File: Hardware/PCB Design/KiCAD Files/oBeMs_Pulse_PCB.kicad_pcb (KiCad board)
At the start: 2 copper layers, 180.3 x 120.7 mm, 132 parts, among them P1 1WIRE_OUT, P10 5V, P11 3V3, P12 GND, P13 ADC_0-7, P14 ADC_8-15, P15 ADC_VREF_2, P16 ADC_VREF_1, P17 SPI_ADC_DAC, P18 DIO_OUTPUT, P19 PULL_UP, P2 1WIRE_SENSOR, P20 PULL_DOWN, P21 DIO_INPUT, P22 DIO_OUTPUT, P23 PULL_UP, P24 PULL_DOWN, P25 DIO_INPUT, P26 DIO_OUTPUT, P27 PULL_UP, P28 PULL_DOWN, P29 DIO_INPUT, P3 HARD_WDT, P34 DAC_A, P35 DAC_B, P36 PROTOTYPING_AREA, P4 LED 5-8, P6 AC_INPUT, P7 LED 1-4, P8 VIN_DC, Q1 BC546, Q2 BC556, U1 LM2575, U2 DS18B20, U3 TLC555, U4 4017, U5 MCP3008, U6 MCP3008, U7 MCP4802, U8 LM2576

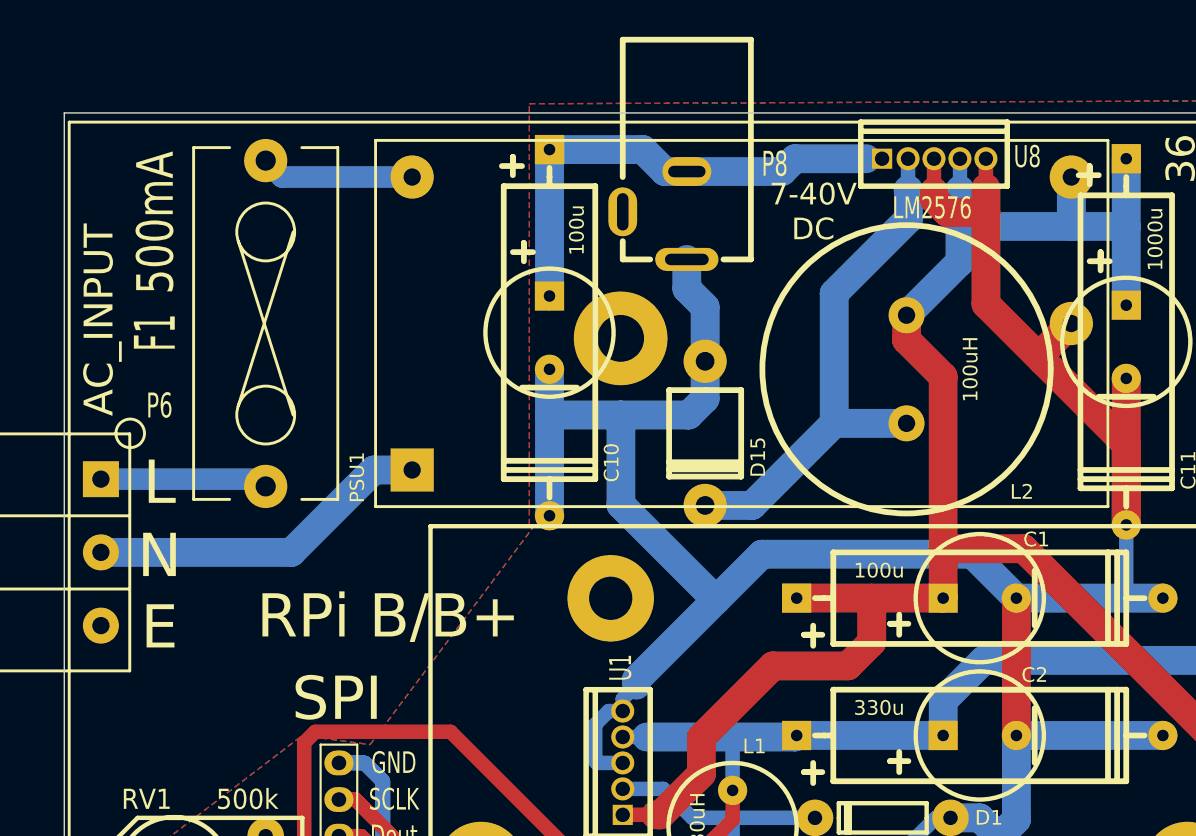
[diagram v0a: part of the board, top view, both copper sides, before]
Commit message: Updated small changes.
Info and changes from email 18/12/15.
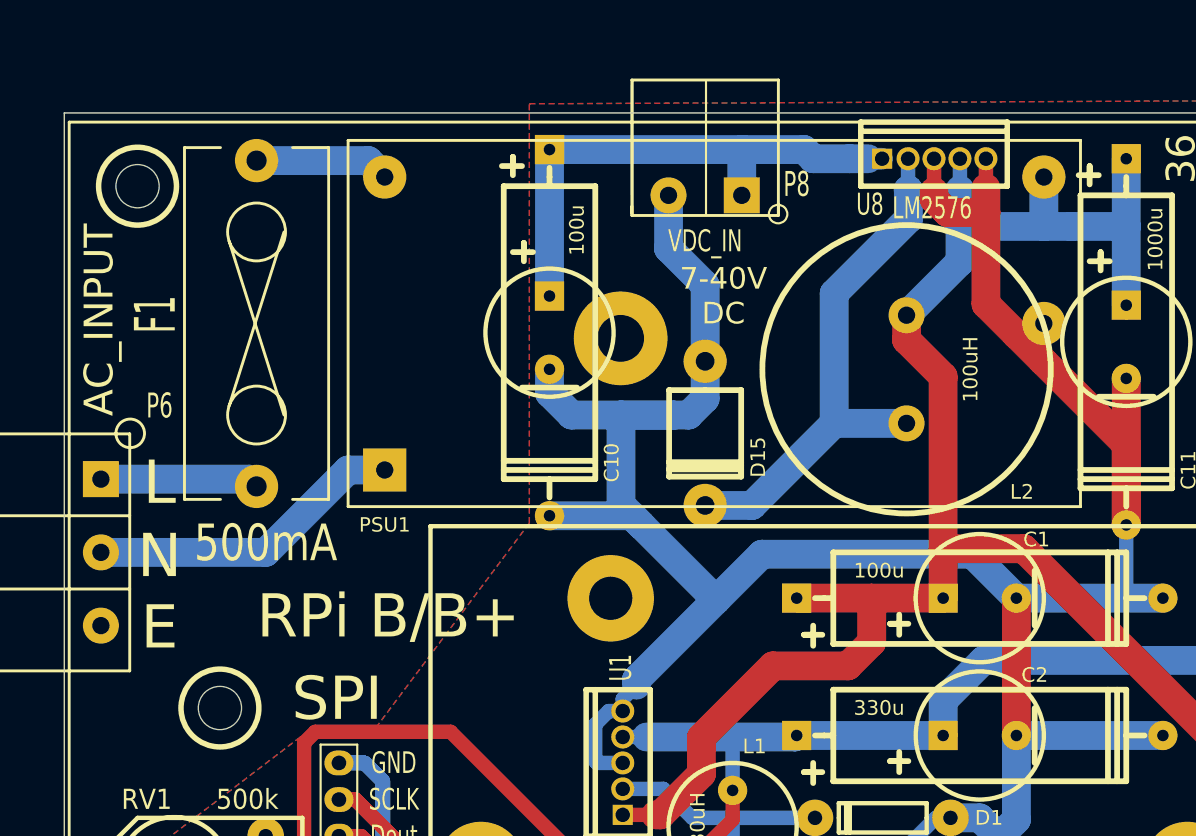
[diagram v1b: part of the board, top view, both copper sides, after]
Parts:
- added H1: Bolt Hole, REInnovationFootprint:3mm_hole, F.Cu at (83.2, 76.8)
- added H2: Bolt Hole, REInnovationFootprint:3mm_hole, F.Cu at (77.5, 40.6)
- L2: footprint TH_Inductor_ELC18B101L -> REInnovationFootprint:TH_Inductor_ELC18B101L
- P8: value VIN_DC -> VDC_IN; footprint REInnovationFootprint:DC_Power_2_1 -> REInnovationFootprint:TH_CONN_2W
- moved P8 4.62 mm to (114.3, 41.3)
- moved PSU1 1.91 mm to (117.5, 50.2)
- moved F1 0.64 mm to (85.7, 50.2)
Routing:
- net GND: track 1033.7 -> 1012.9 mm
- net /PowerSupply/VDC_IN+: track 52.3 -> 48.2 mm
- net /PowerSupply/N: track 24.0 -> 22.1 mm
- net Net-(F1-Pad2): track 10.6 -> 9.36 mm
- net +5V: track 193.4 -> 193.9 mm

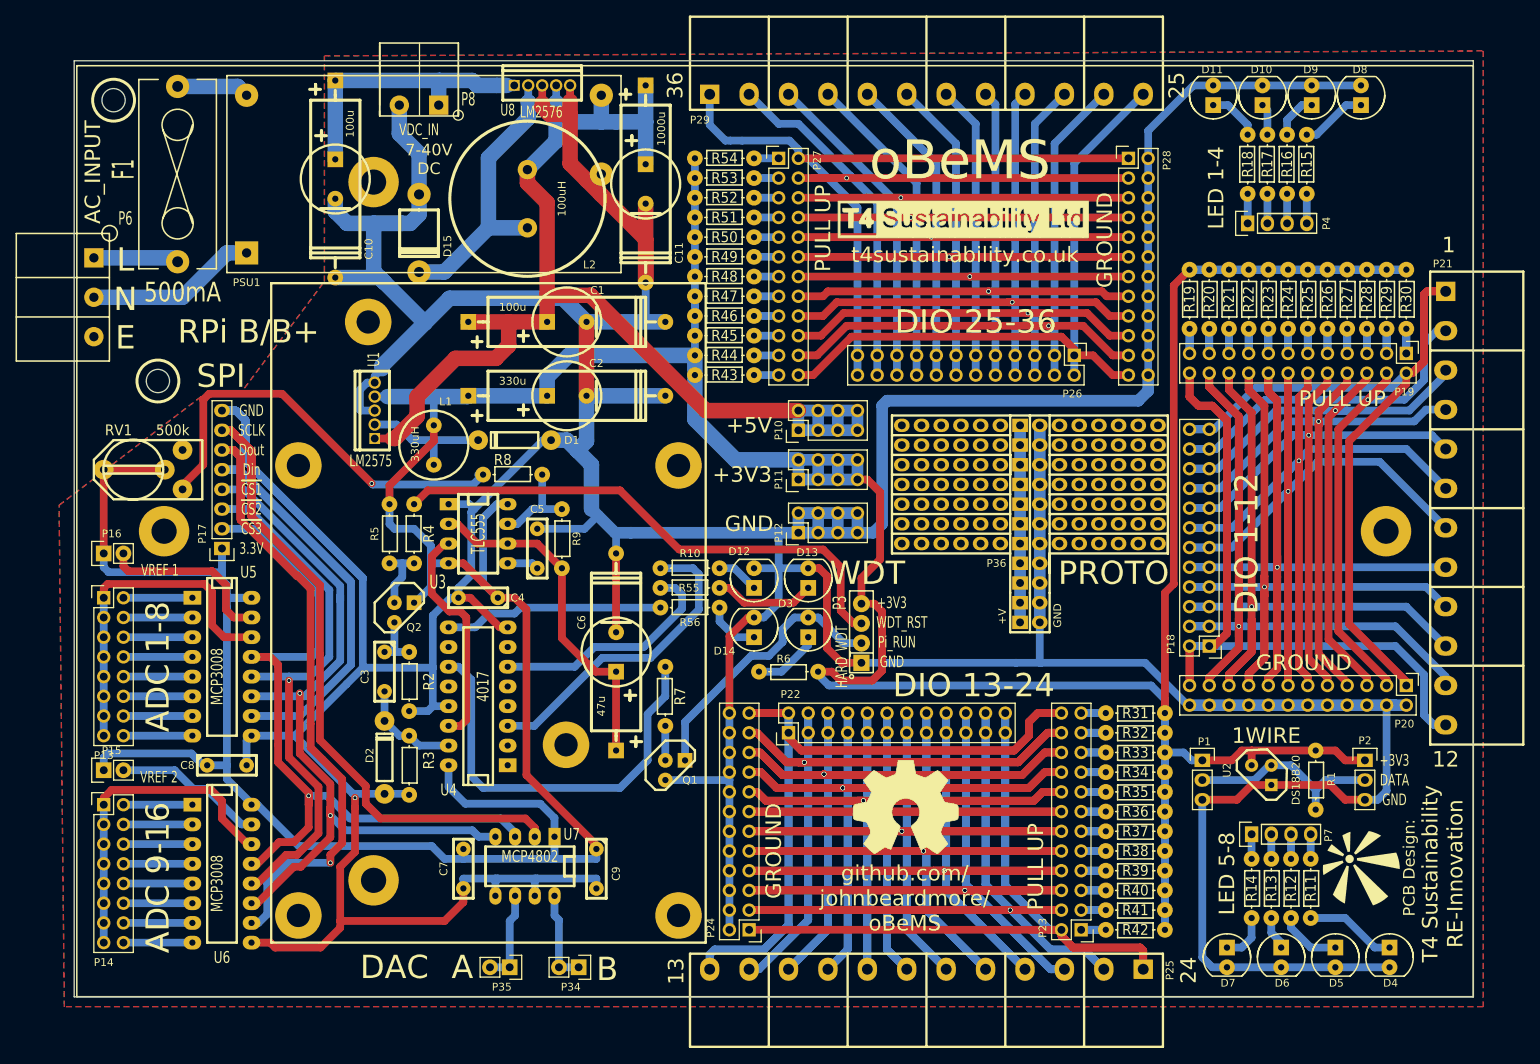
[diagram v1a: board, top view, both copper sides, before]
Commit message: Small changes on PCB
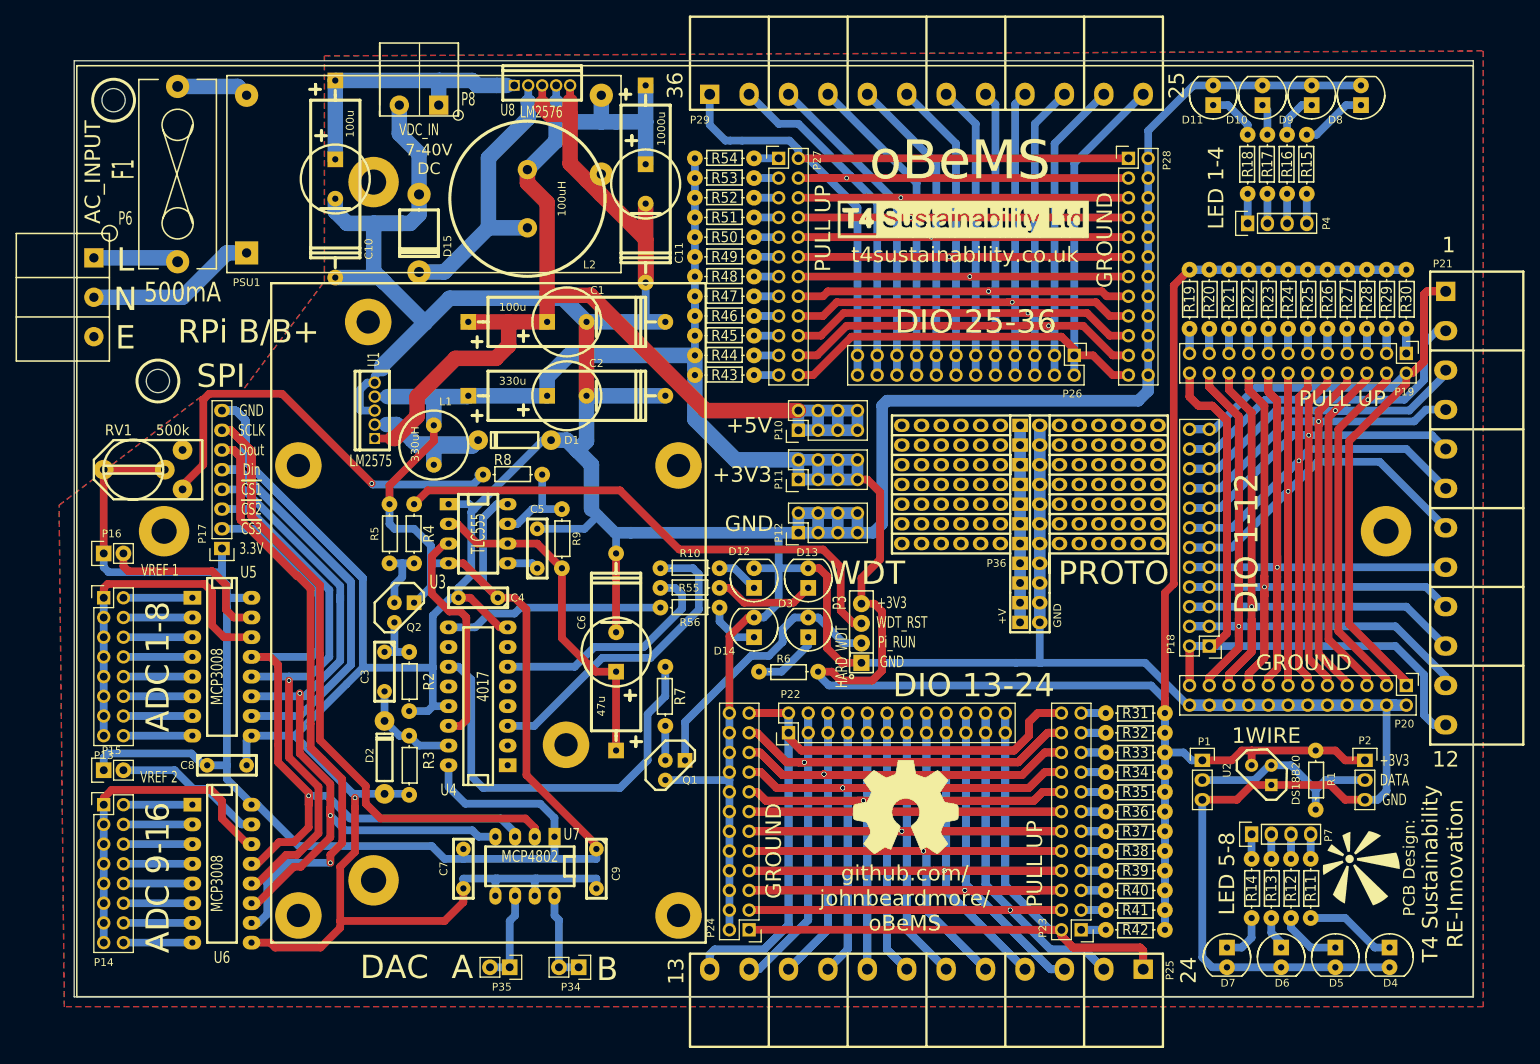
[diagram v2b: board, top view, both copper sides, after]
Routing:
- net Net-(D1-Pad2): track 17.9 -> 32.3 mm
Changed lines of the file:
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@@
     (thickness 1.6)
     (drawings 60)
-    (tracks 1615)
+    (tracks 1622)
     (zones 0)
     (modules 134)
@@
     (tags "LED led 5mm 5MM 100mil 2,54mm")
     (attr virtual)
-    (fp_text reference D11 (at 3.302 -0.127 180) (layer F.SilkS)
+    (fp_text reference D11 (at -3.175 -2.667 180) (layer F.SilkS)
       (effects (font (size 1 1) (thickness 0.15)))
     )
@@
     (tags "LED led 5mm 5MM 100mil 2,54mm")
     (attr virtual)
-    (fp_text reference D10 (at 3.302 -0.127 180) (layer F.SilkS)
+    (fp_text reference D10 (at -3.175 -3.302 180) (layer F.SilkS)
       (effects (font (size 1 1) (thickness 0.15)))
     )
@@
     (tags "LED led 5mm 5MM 100mil 2,54mm")
     (attr virtual)
-    (fp_text reference D9 (at 3.302 -0.127 180) (layer F.SilkS)
+    (fp_text reference D9 (at -3.175 -3.302 180) (layer F.SilkS)
       (effects (font (size 1 1) (thickness 0.15)))
     )
@@
     (tags "LED led 5mm 5MM 100mil 2,54mm")
     (attr virtual)
-    (fp_text reference D8 (at 3.302 -0.127 180) (layer F.SilkS)
+    (fp_text reference D8 (at -3.175 -3.302 180) (layer F.SilkS)
       (effects (font (size 1 1) (thickness 0.15)))
     )
@@
     (effects (font (size 2 2) (thickness 0.5)))
   )
-  (gr_text "PULL UP" (at 196.342 139.446 90) (layer F.SilkS)
+  (gr_text "PULL UP" (at 196.215 139.065 90) (layer F.SilkS)
     (effects (font (size 2 2) (thickness 0.5)))
   )
@@
     (effects (font (size 3 3) (thickness 0.75)))
   )
+  (segment (start 118.745 82.55) (end 118.745 78.845) (width 2) (layer B.Cu) (net 1))
   (segment (start 152.4 73.533) (end 152.4 81.788) (width 2) (layer B.Cu) (net 1))
   (segment (start 157.607 86.995) (end 165.735 86.995) (width 2) (layer B.Cu) (net 1))
@@
   (segment (start 152.4 81.026) (end 158.369 86.995) (width 1) (layer B.Cu) (net 1))
   (segment (start 158.369 86.995) (end 165.735 86.995) (width 1) (layer B.Cu) (net 1))
-  (segment (start 118.745 82.55) (end 118.745 78.845) (width 1) (layer B.Cu) (net 1))
   (segment (start 118.745 78.845) (end 119.126 78.845) (width 1) (layer B.Cu) (net 1))
   (segment (start 111.125 78.845) (end 112.776 78.845) (width 1) (layer B.Cu) (net 1))
@@
   (segment (start 124.333 97.79) (end 128.27 97.79) (width 1) (layer F.Cu) (net 22))
   (segment (start 121.793 95.25) (end 124.333 97.79) (width 1) (layer F.Cu) (net 22))
+  (segment (start 118.745 85.217) (end 118.745 87.63) (width 2) (layer B.Cu) (net 23))
+  (segment (start 112.649 82.445) (end 113.941 82.445) (width 2) (layer B.Cu) (net 23))
+  (segment (start 113.941 82.445) (end 115.951 84.455) (width 2) (layer B.Cu) (net 23))
+  (segment (start 115.951 84.455) (end 116.713 85.217) (width 2) (layer B.Cu) (net 23))
+  (segment (start 116.713 85.217) (end 118.745 85.217) (width 2) (layer B.Cu) (net 23))
+  (segment (start 118.745 85.217) (end 123.698 85.217) (width 2) (layer B.Cu) (net 23))
+  (segment (start 123.698 85.217) (end 124.46 84.455) (width 2) (layer B.Cu) (net 23))
   (segment (start 118.745 87.63) (end 118.745 84.455) (width 1) (layer B.Cu) (net 23))
-  (segment (start 111.125 82.445) (end 113.941 82.445) (width 1) (layer B.Cu) (net 23))
+  (segment (start 111.125 82.445) (end 112.649 82.445) (width 1) (layer B.Cu) (net 23))
   (segment (start 115.951 84.455) (end 118.745 84.455) (width 1) (layer B.Cu) (net 23))
   (segment (start 118.745 84.455) (end 124.46 84.455) (width 1) (layer B.Cu) (net 23))
